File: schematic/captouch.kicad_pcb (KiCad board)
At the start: 2 copper layers, 26 x 40 mm, 13 parts, among them P1 CONN_01X02, P2 CONN_01X04, P3 CONN_01X03, Q1 DMN3404L, U1 LD1117S33CTR, U2 MSP430G2553IPW20

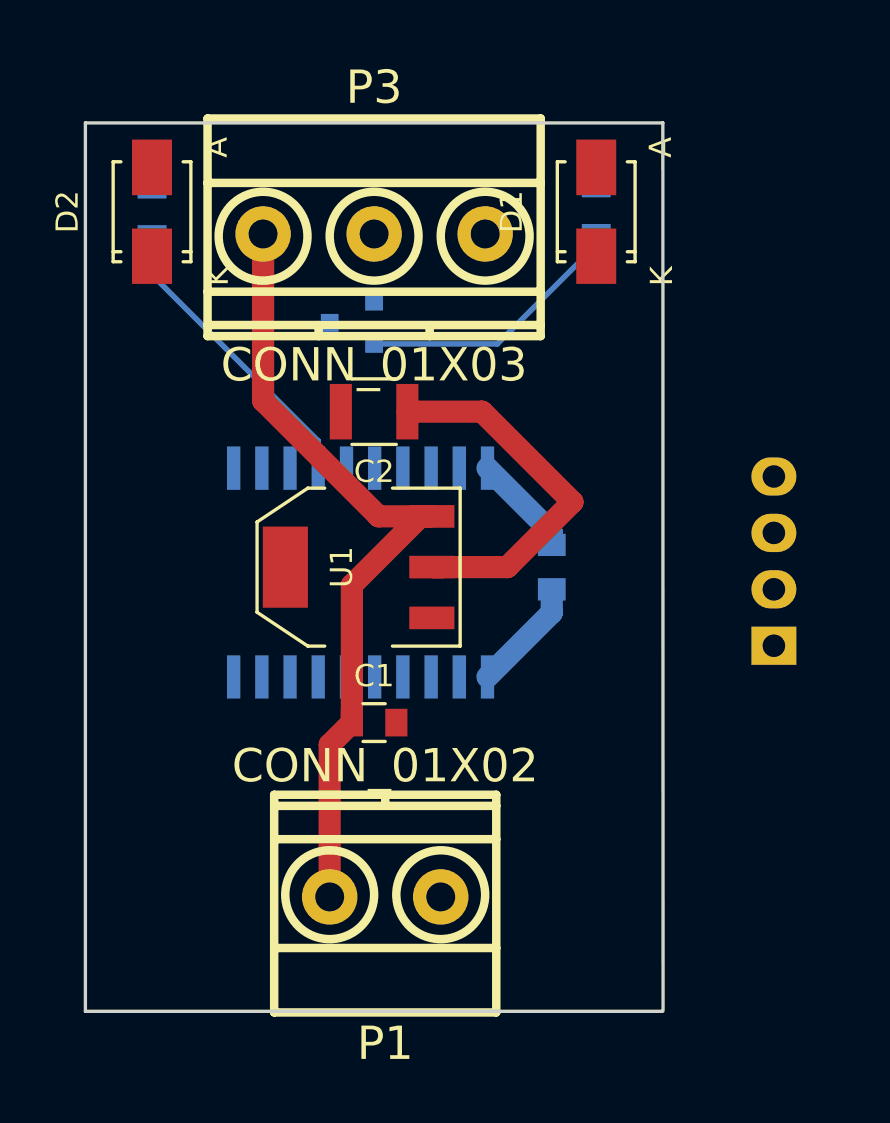
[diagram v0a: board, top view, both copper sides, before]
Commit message: Finished routing
Artwork is next
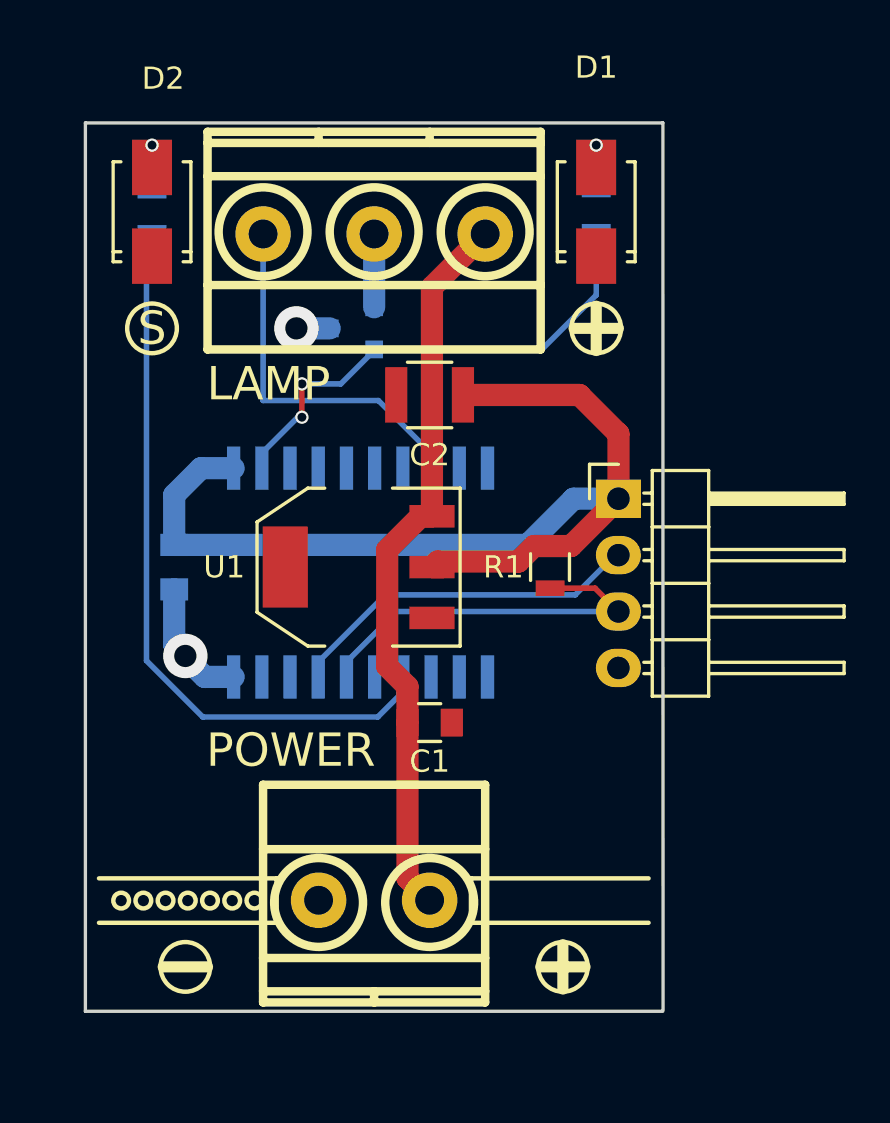
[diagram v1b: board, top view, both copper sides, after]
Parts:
- added R1: 47k, Resistors_SMD:R_0805, F.Cu at (72.9, 55.0)
- P1: value CONN_01X02 -> POWER
- P2: value CONN_01X04 -> PROG; moved to F.Cu
- P3: value CONN_01X03 -> LAMP
- moved C3 17.0 mm to (56.0, 55.0), turned to 270 degrees
- moved P2 9.63 mm to (76.0, 51.9)
- moved C2 2.61 mm to (67.5, 47.2)
- moved C1 2.50 mm to (67.5, 62.0)
- moved P1 0.52 mm to (65.0, 70.0), turned to 0 degrees
- moved Q1 0.25 mm to (64.0, 44.2)
- turned P3 to 180 degrees
- turned U2 to 270 degrees
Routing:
- net +3V3: track 22.3 -> 47.1 mm
- net Net-(R3-Pad2): track 13.7 -> 33.1 mm
- net Net-(P3-Pad3): track 0.00 -> 16.7 mm
- net /RST: track 0.67 -> 17.4 mm
- net TEST: track 0.67 -> 16.2 mm
- net Net-(Q1-Pad2): track 12.4 -> 22.4 mm, vias 0 -> 2
- net Net-(C1-Pad1): track 36.6 -> 32.9 mm
- net Net-(P3-Pad2): track 0.00 -> 3.30 mm
- net Net-(D2-Pad2): track 0.00 -> 3.05 mm, vias 0 -> 1
- net Net-(D1-Pad2): track 0.00 -> 3.00 mm, vias 0 -> 1
- net GNDREF: track 4.65 -> 7.32 mm, vias 0 -> 2
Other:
- board text added: "S"
